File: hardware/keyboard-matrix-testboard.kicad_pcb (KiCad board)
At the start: 2 copper layers, 38 x 32 mm, 87 parts, among them J1 USB_B_Micro, J2 EZmate-3, J3 EZmate-4, J5 TC2030-IDC-NL, Q1 BSS84, SW1 SW_Push, SW10 SW_Push, SW11 SW_Push, SW12 SW_Push, SW13 SW_Push, SW14 SW_Push, SW15 SW_Push, SW16 SW_Push, SW17 SW_Push, SW18 SW_Push, SW19 SW_Push, SW2 SW_Push, SW20 SW_Push, SW3 SW_Push, SW4 SW_Push, SW5 SW_Push, SW6 SW_Push, SW7 SW_Push, SW8 SW_Push, SW9 SW_Push, U1 STBC08, U2 nRF52832-QFxx, U3 MIC5301, U4 PCAL6408A, Y1 32.768kHz, Y2 32MHz

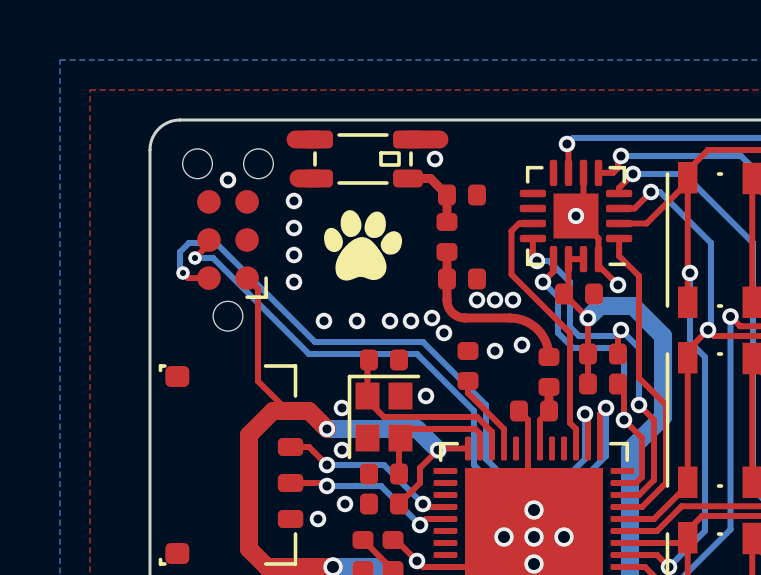
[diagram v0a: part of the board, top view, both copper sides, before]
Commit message: hw: r0
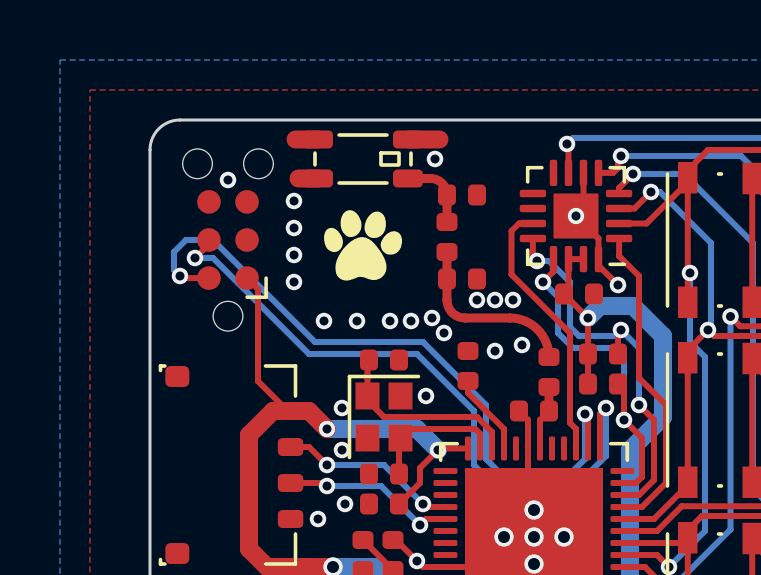
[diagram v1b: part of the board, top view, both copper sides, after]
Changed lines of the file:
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@@
   (segment (start 118.9 81.4) (end 118.9 80.5) (width 0.3) (layer "F.Cu") (net 1))
   (segment (start 118.35 79.95) (end 117.6 79.95) (width 0.3) (layer "F.Cu") (net 1))
-  (segment (start 118.9 80.5) (end 118.35 79.95) (width 0.3) (layer "F.Cu") (net 1))
+  (arc (start 118.9 80.5) (mid 118.738909 80.111091) (end 118.35 79.95) (width 0.3) (layer "F.Cu") (net 1))
   (segment (start 121.6 91.2) (end 121.6 91.7) (width 0.2) (layer "F.Cu") (net 2))
   (segment (start 117.9 92.7) (end 117.2 92) (width 0.2) (layer "F.Cu") (net 2))
@@
   (segment (start 123.6 87.9) (end 123.6 88.95) (width 0.2) (layer "F.Cu") (net 50))
   (segment (start 123.5 87.8) (end 123.6 87.9) (width 0.2) (layer "F.Cu") (net 50))
-  (segment (start 110.27 83.27) (end 110.965 83.27) (width 0.2) (layer "F.Cu") (net 50))
-  (segment (start 110.1 83.1) (end 110.27 83.27) (width 0.2) (layer "F.Cu") (net 50))
+  (segment (start 110 83.2) (end 110.07 83.27) (width 0.2) (layer "F.Cu") (net 50))
+  (segment (start 110.07 83.27) (end 110.965 83.27) (width 0.2) (layer "F.Cu") (net 50))
+  (via (at 110 83.2) (size 0.55) (drill 0.3) (layers "F.Cu" "B.Cu") (net 50))
   (via (at 123.5 87.8) (size 0.55) (drill 0.3) (layers "F.Cu" "B.Cu") (net 50))
-  (via (at 110.1 83.1) (size 0.45) (drill 0.2) (layers "F.Cu" "B.Cu") (net 50))
+  (segment (start 123.5 89.3) (end 123.5 87.8) (width 0.2) (layer "B.Cu") (net 50))
+  (segment (start 109.8 83) (end 109.8 82.4) (width 0.2) (layer "B.Cu") (net 50))
+  (segment (start 120.2 87.5) (end 120.2 89.3) (width 0.2) (layer "B.Cu") (net 50))
+  (segment (start 111.1 82) (end 114.5 85.4) (width 0.2) (layer "B.Cu") (net 50))
+  (segment (start 123 89.8) (end 123.5 89.3) (width 0.2) (layer "B.Cu") (net 50))
+  (segment (start 109.8 82.4) (end 110.2 82) (width 0.2) (layer "B.Cu") (net 50))
+  (segment (start 110.2 82) (end 111.1 82) (width 0.2) (layer "B.Cu") (net 50))
+  (segment (start 120.2 89.3) (end 120.7 89.8) (width 0.2) (layer "B.Cu") (net 50))
+  (segment (start 110 83.2) (end 109.8 83) (width 0.2) (layer "B.Cu") (net 50))
   (segment (start 120.7 89.8) (end 123 89.8) (width 0.2) (layer "B.Cu") (net 50))
-  (segment (start 110 83) (end 110 82.4) (width 0.2) (layer "B.Cu") (net 50))
+  (segment (start 118.1 85.4) (end 120.2 87.5) (width 0.2) (layer "B.Cu") (net 50))
   (segment (start 114.5 85.4) (end 118.1 85.4) (width 0.2) (layer "B.Cu") (net 50))
-  (segment (start 111.2 82.1) (end 114.5 85.4) (width 0.2) (layer "B.Cu") (net 50))
-  (segment (start 120.2 89.3) (end 120.7 89.8) (width 0.2) (layer "B.Cu") (net 50))
-  (segment (start 110.1 83.1) (end 110 83) (width 0.2) (layer "B.Cu") (net 50))
-  (segment (start 123.5 89.3) (end 123.5 87.8) (width 0.2) (layer "B.Cu") (net 50))
-  (segment (start 118.1 85.4) (end 120.2 87.5) (width 0.2) (layer "B.Cu") (net 50))
-  (segment (start 110.3 82.1) (end 111.2 82.1) (width 0.2) (layer "B.Cu") (net 50))
-  (segment (start 110 82.4) (end 110.3 82.1) (width 0.2) (layer "B.Cu") (net 50))
-  (segment (start 120.2 87.5) (end 120.2 89.3) (width 0.2) (layer "B.Cu") (net 50))
-  (segment (start 123 89.8) (end 123.5 89.3) (width 0.2) (layer "B.Cu") (net 50))
   (segment (start 124.2 87.6) (end 124 87.8) (width 0.2) (layer "F.Cu") (net 51))
   (segment (start 110.5 82.6) (end 110.965 82.135) (width 0.2) (layer "F.Cu") (net 51))
@@
   (segment (start 124 87.8) (end 124 88.95) (width 0.2) (layer "F.Cu") (net 51))
   (via (at 124.2 87.6) (size 0.55) (drill 0.3) (layers "F.Cu" "B.Cu") (net 51))
-  (via (at 110.5 82.6) (size 0.45) (drill 0.2) (layers "F.Cu" "B.Cu") (net 51))
+  (via (at 110.5 82.6) (size 0.55) (drill 0.3) (layers "F.Cu" "B.Cu") (net 51))
   (segment (start 123.2 90.2) (end 124.2 89.2) (width 0.2) (layer "B.Cu") (net 51))
   (segment (start 114.3 85.8) (end 117.9 85.8) (width 0.2) (layer "B.Cu") (net 51))
